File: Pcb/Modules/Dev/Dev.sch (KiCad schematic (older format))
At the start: 8 parts, among them J1 JACK_STEREO, J2 JACK_RJ45, P1 CONN_02X04, P2 CONN_02X04, Q1 Q_NMOS_GSD

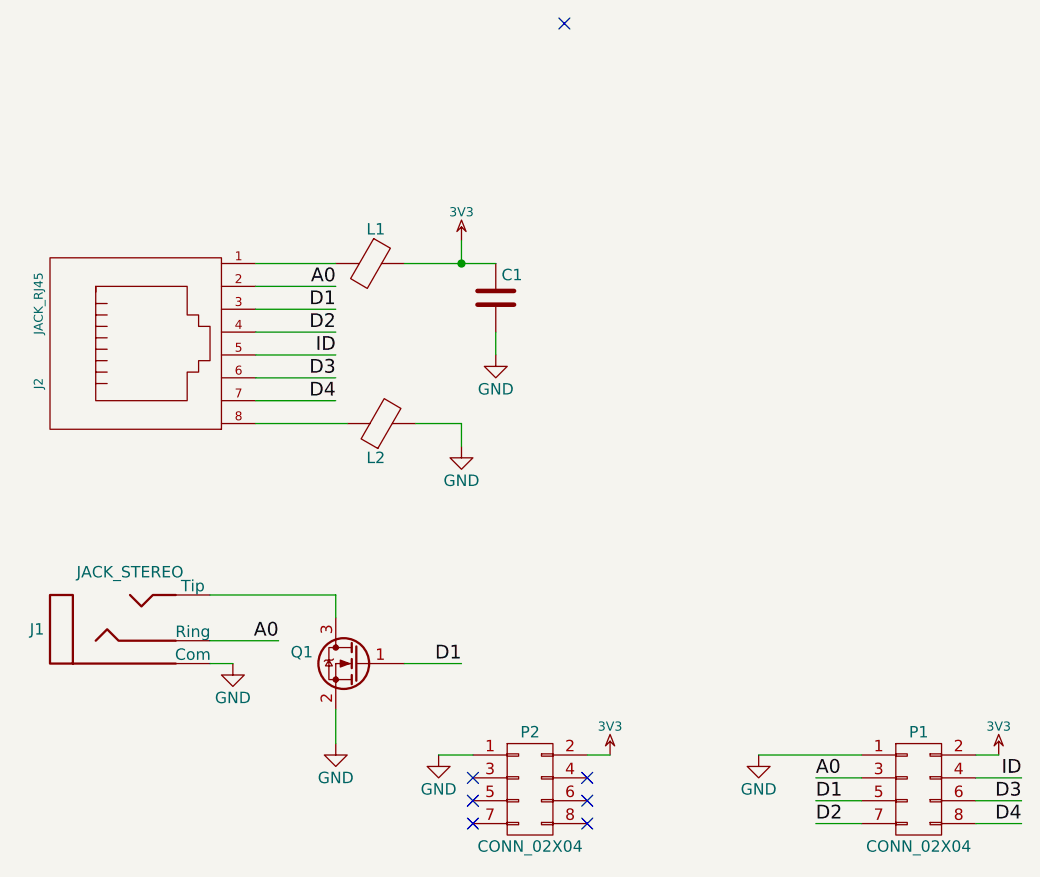
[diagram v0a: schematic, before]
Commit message: Update dev module pcb
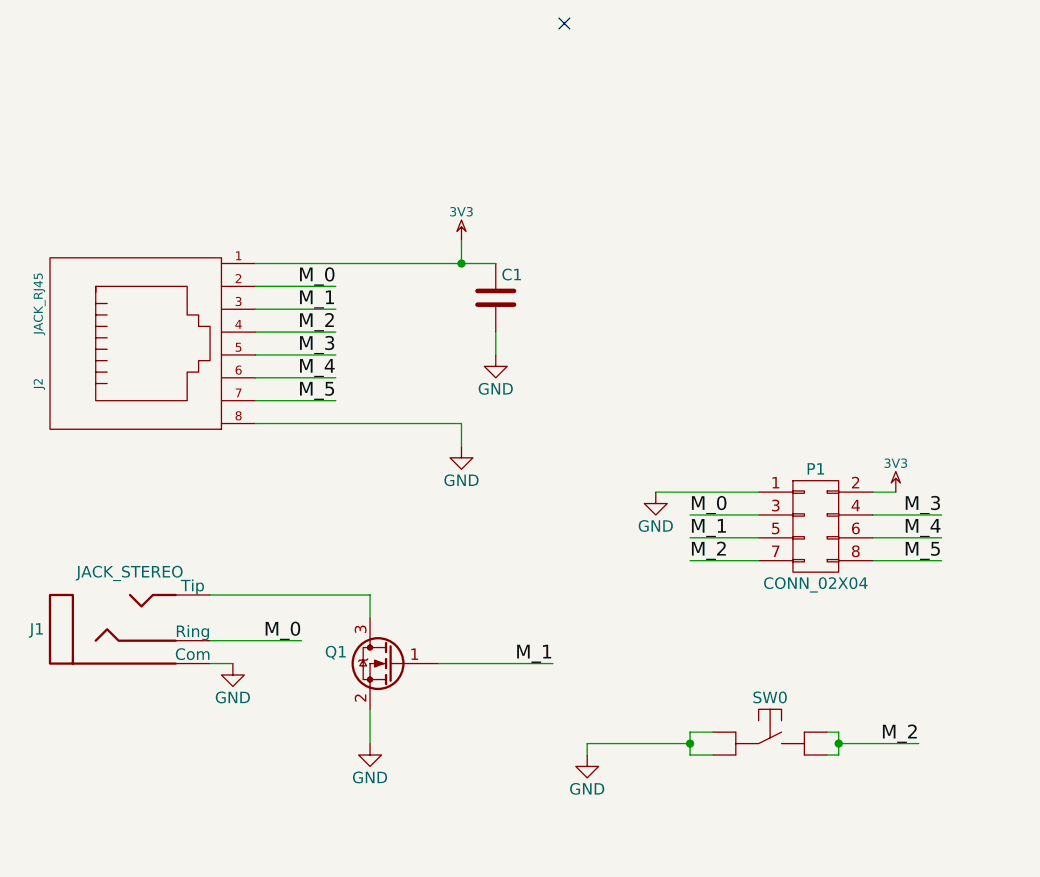
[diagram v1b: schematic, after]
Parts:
- removed L1, L2: Ferrite_Bead, Resistors_SMD:R_0805, symbol Ferrite_Bead
- removed P2: CONN_02X04, Socket_Strips:Socket_Strip_Straight_2x04_Pitch2.54mm, symbol CONN_02X04
- added SW0: SW_TACTILE, CA6:PTS645, symbol SW_TACTILE
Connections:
- net 3V3: now also J2.1
- net GND: now also J2.8, SW0.1, SW0.2
- net A0 renamed M_0
- net D1 renamed M_1
- net D2 renamed M_2
- net M_2: now also SW0.3, SW0.4
- net D3 renamed M_4
- net D4 renamed M_5
- net ID renamed M_3
- no-connect marks 7 -> 1
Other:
- moved on the sheet: P1, Q1
